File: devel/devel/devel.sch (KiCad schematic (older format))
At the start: 1 part

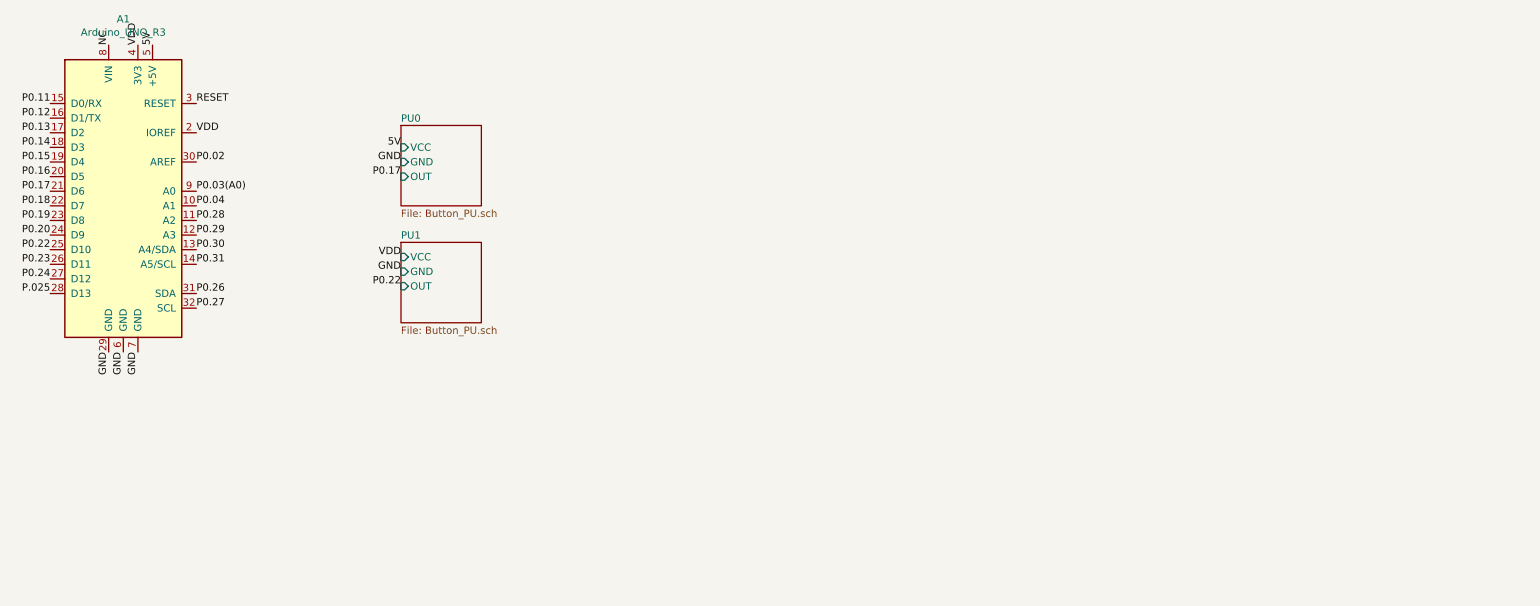
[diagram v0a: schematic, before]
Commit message: Worked on the dev-board
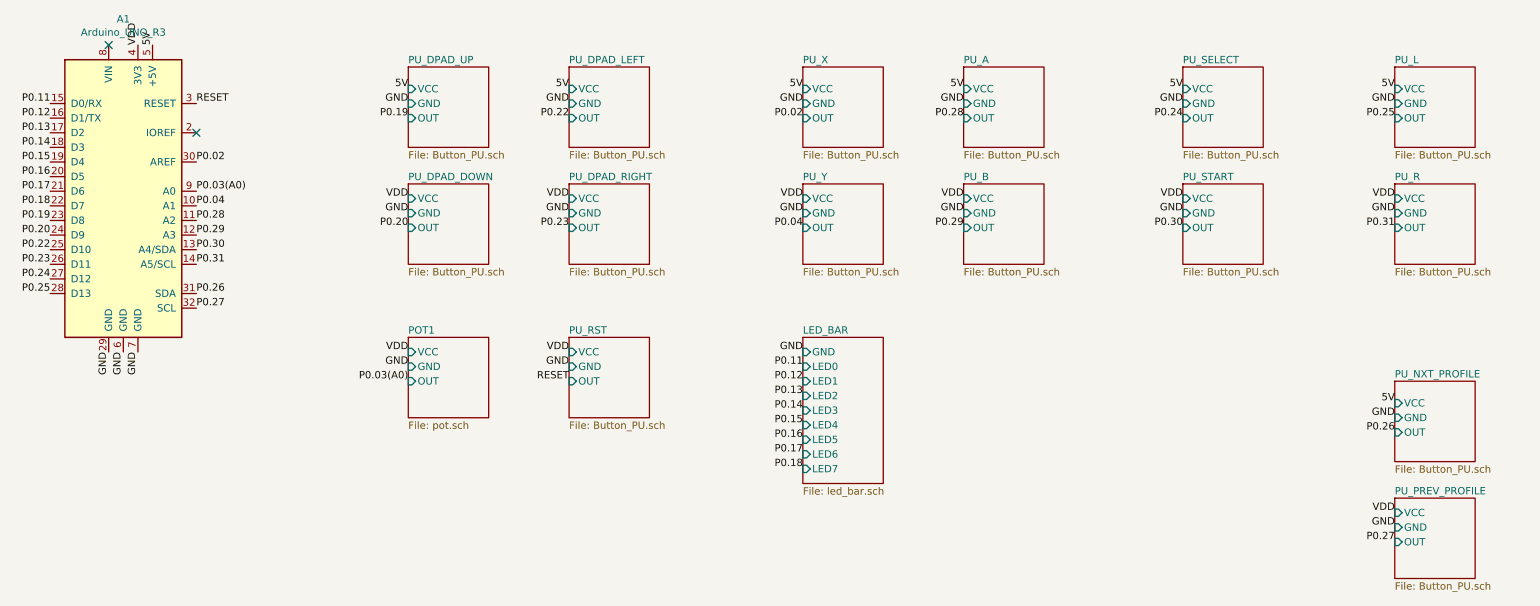
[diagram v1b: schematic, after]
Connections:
- net VDD: no longer A1.2 (IOREF)
- net NC: no longer names the net of A1.8 (VIN)
- net P.025 renamed P0.25
- no-connect marks 0 -> 2
